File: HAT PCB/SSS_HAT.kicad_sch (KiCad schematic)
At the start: 23 parts, among them J1 ESP32_Connector_0, J2 ESP32_Connector_1, J3 CAN, J4 CAN, J5 I2C, J6 ADC, U1 TJA1051T, U2 ADS8320EB_250, U3 ICM-42688-P

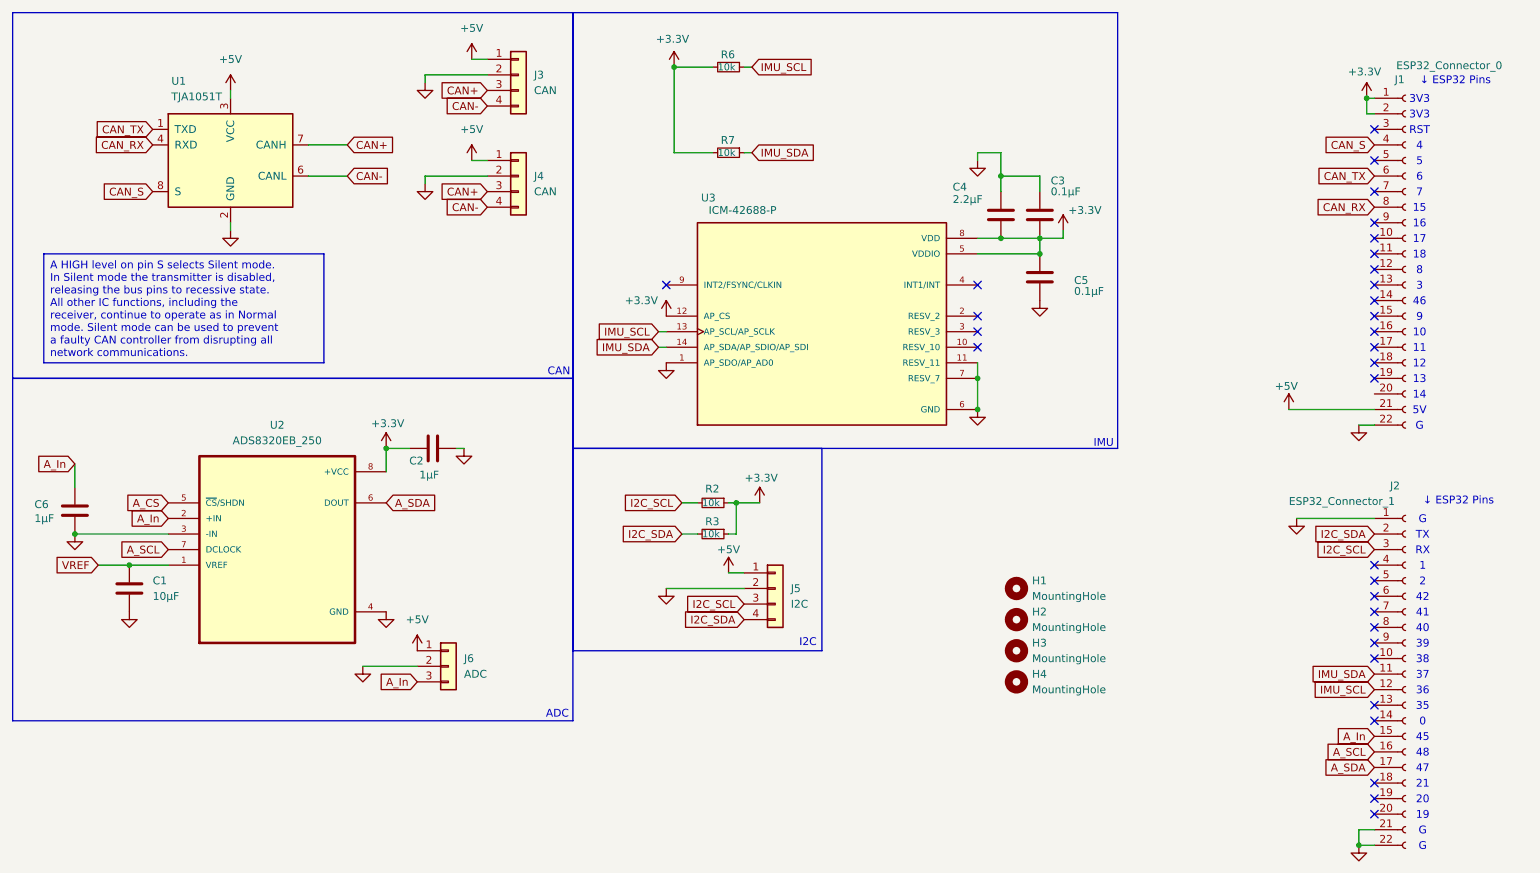
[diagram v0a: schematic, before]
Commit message: Updated 3D model & readme.
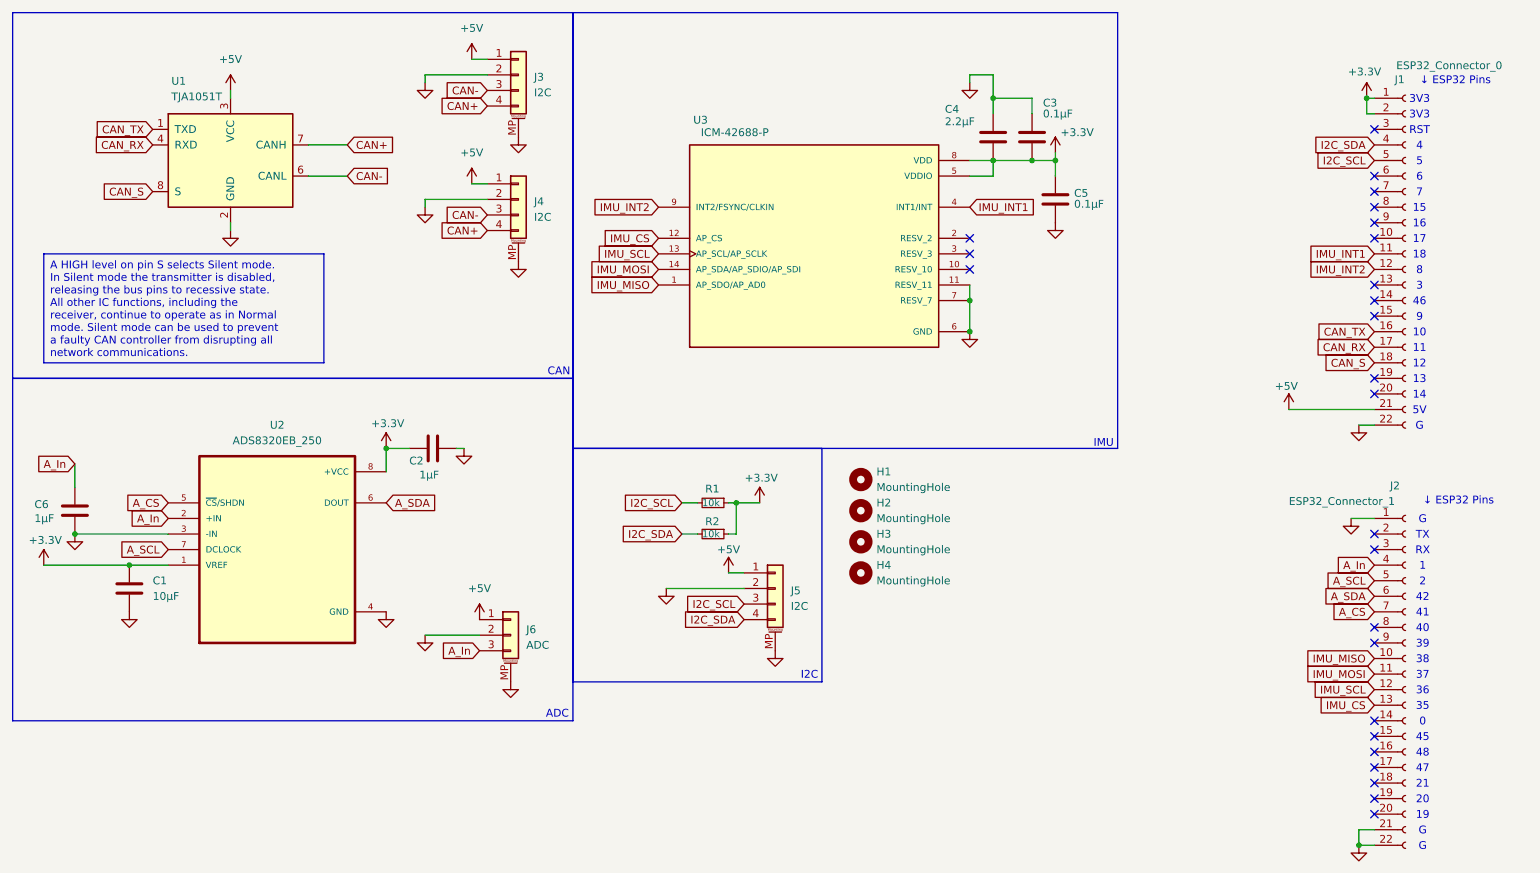
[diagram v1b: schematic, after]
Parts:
- removed J3, J4: CAN, Connector_Molex:Molex_Nano-Fit_105313-xx04_1x04_P2.50mm_Horizontal, symbol Connector_Generic:Conn_01x04
- removed J5: I2C, Connector_Molex:Molex_Nano-Fit_105313-xx04_1x04_P2.50mm_Horizontal, symbol Connector_Generic:Conn_01x04
- removed J6: ADC, symbol Connector_Generic:Conn_01x03
- removed R6, R7: 10k, Resistor_SMD:R_0402_1005Metric_Pad0.72x0.64mm_HandSolder, symbol Device:R_Small
- added J3, J4, J5: I2C, Connector_Hirose:Hirose_DF3EA-04P-2H_1x04-1MP_P2.00mm_Horizontal, symbol Connector_Generic_MountingPin:Conn_01x04_MountingPin
- added J6: ADC, Connector_Hirose:Hirose_DF3EA-03P-2H_1x03-1MP_P2.00mm_Horizontal, symbol Connector_Generic_MountingPin:Conn_01x03_MountingPin
- C1, C2, C6: footprint (none) -> Capacitor_SMD:C_0402_1005Metric_Pad0.74x0.62mm_HandSolder
- U2: footprint ADS8320EB_250:SOP65P490X110-8N -> ADS8320EB_250:DGK0008A_L
- renumbered R2 to R1, R3 to R2
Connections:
- net VREF is gone; now on net +3.3V: C1.1, U2.1 (VREF)
- net +3.3V: no longer U3.12 (AP_CS)
- net +5V: now also J3.1 (Pin_1), J4.1 (Pin_1), J5.1 (Pin_1), J6.1 (Pin_1)
- net A_CS: now also J2.7 (Pin_7)
- net A_In: now also J2.4 (Pin_4), J6.3 (Pin_3); no longer J2.15 (Pin_15)
- net A_SCL: now also J2.5 (Pin_5); no longer J2.16 (Pin_16)
- net A_SDA: now also J2.6 (Pin_6); no longer J2.17 (Pin_17)
- net CAN+: now also J3.4 (Pin_4), J4.4 (Pin_4)
- net CAN-: now also J3.3 (Pin_3), J4.3 (Pin_3)
- net CAN_RX: now also J1.17 (Pin_17); no longer J1.8 (Pin_8)
- net CAN_S: now also J1.18 (Pin_18); no longer J1.4 (Pin_4)
- net CAN_TX: now also J1.16 (Pin_16); no longer J1.6 (Pin_6)
- net GND: now also J3.2 (Pin_2), J3.MP (MountPin), J4.2 (Pin_2), J4.MP (MountPin), J5.2 (Pin_2), J5.MP (MountPin), J6.2 (Pin_2), J6.MP (MountPin); no longer U3.1 (AP_SDO/AP_AD0)
- net I2C_SCL: now also J1.5 (Pin_5), J5.3 (Pin_3); no longer J2.3 (Pin_3)
- net I2C_SDA: now also J1.4 (Pin_4), J5.4 (Pin_4); no longer J2.2 (Pin_2)
- net IMU_INT1: now reaches J1.11 (Pin_11)
- net IMU_INT1: now also U3.4 (INT1/INT)
- net IMU_INT2: now reaches J1.12 (Pin_12)
- net IMU_INT2: now also U3.9 (INT2/FSYNC/CLKIN)
- net IMU_MISO: now reaches J2.10 (Pin_10)
- net IMU_MISO: now also U3.1 (AP_SDO/AP_AD0)
- net IMU_CS: now reaches J2.13 (Pin_13)
- net IMU_CS: now also U3.12 (AP_CS)
- net IMU_SDA renamed IMU_MOSI
- no-connect marks 31 -> 25
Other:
- moved on the sheet: C3, C4, C5, H1, H2, H3, H4, U3
